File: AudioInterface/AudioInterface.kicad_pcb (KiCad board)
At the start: 2 copper layers, 88.1 x 68.3 mm, 29 parts, among them J1 Capsule, J2 Set_Gain, J3 Audio_Out, J4 Power, J5 Conn_02x01_Row_Letter_First, J6 Conn_02x01_Row_Letter_First, U1 THAT1512, U2 NMA0515SC

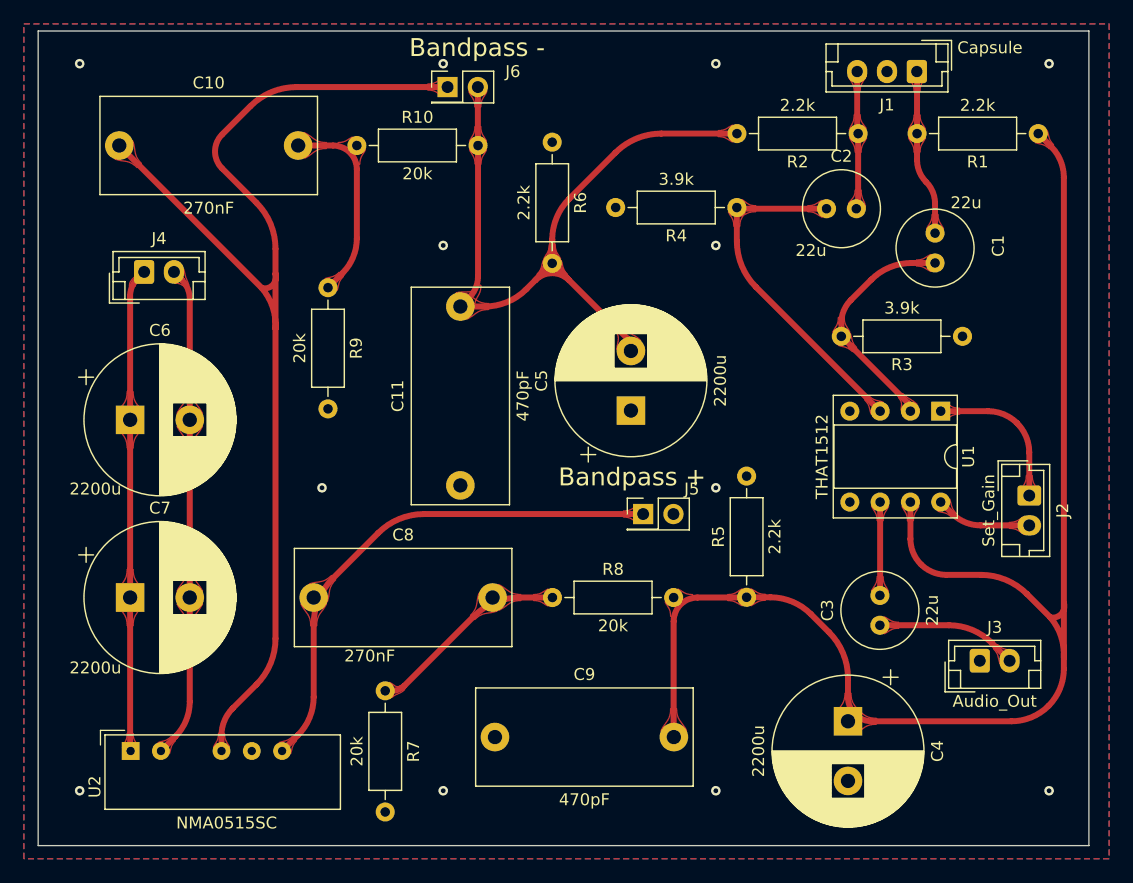
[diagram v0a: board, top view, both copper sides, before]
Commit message: image
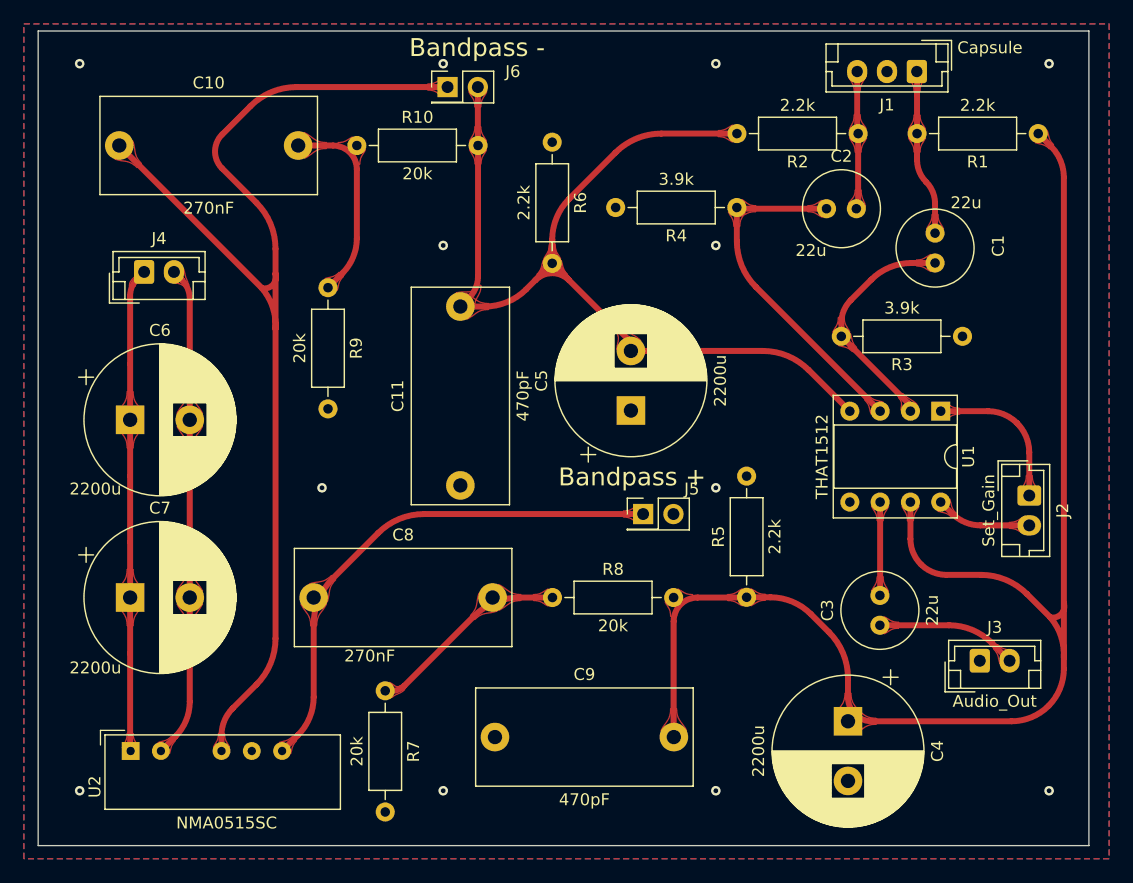
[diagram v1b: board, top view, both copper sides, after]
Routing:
- net /Bandpass-/B_OUT: track 63.2 -> 83.3 mm
